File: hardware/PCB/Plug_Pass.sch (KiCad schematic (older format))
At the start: 14 parts, among them J1 Conn_01x06, J10 TDPT-1017503, J2 Conn_01x08, J3 Conn_01x06, J4 QuickDisconnect, J5 Conn_WallSocket_Earth, J6 QuickDisconnect, J7 Conn_01x06, J8 QuickDisconnect, J9 QuickDisconnect

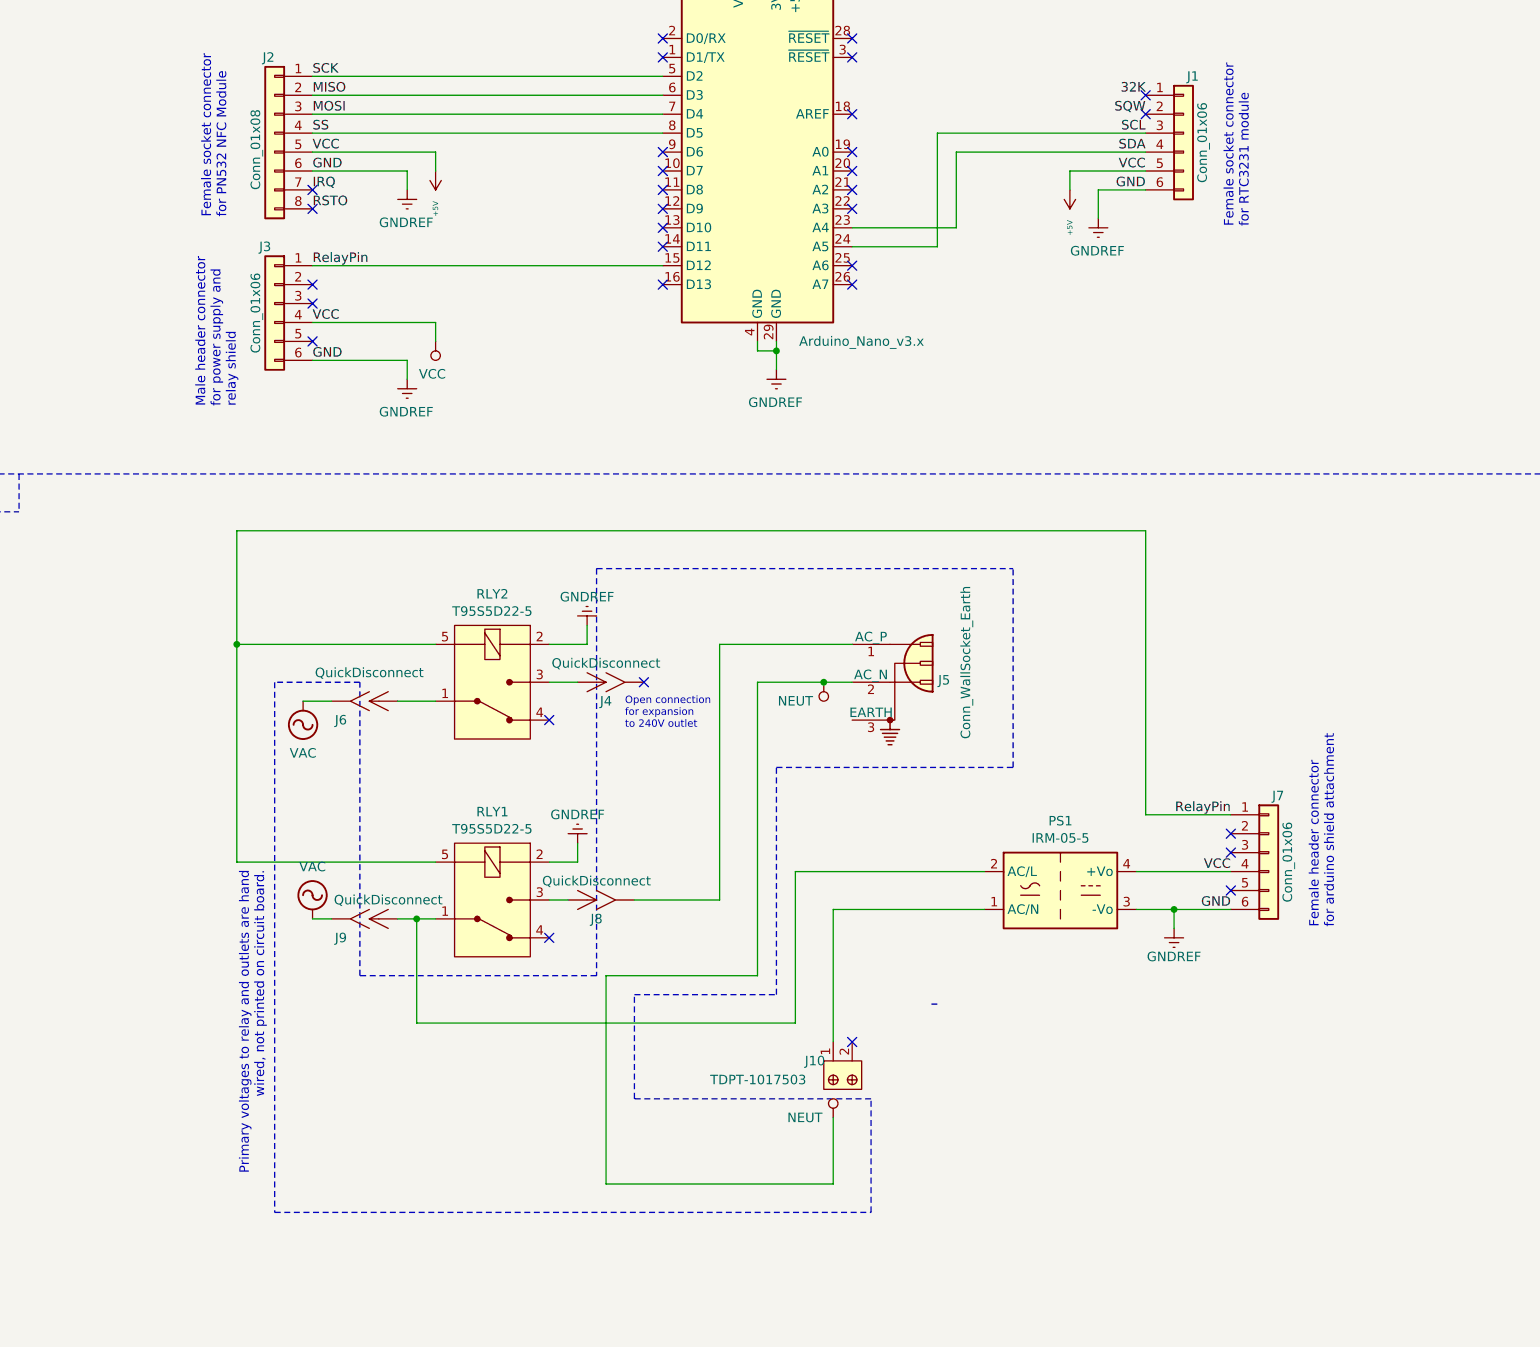
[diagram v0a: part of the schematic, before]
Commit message: Add files via upload
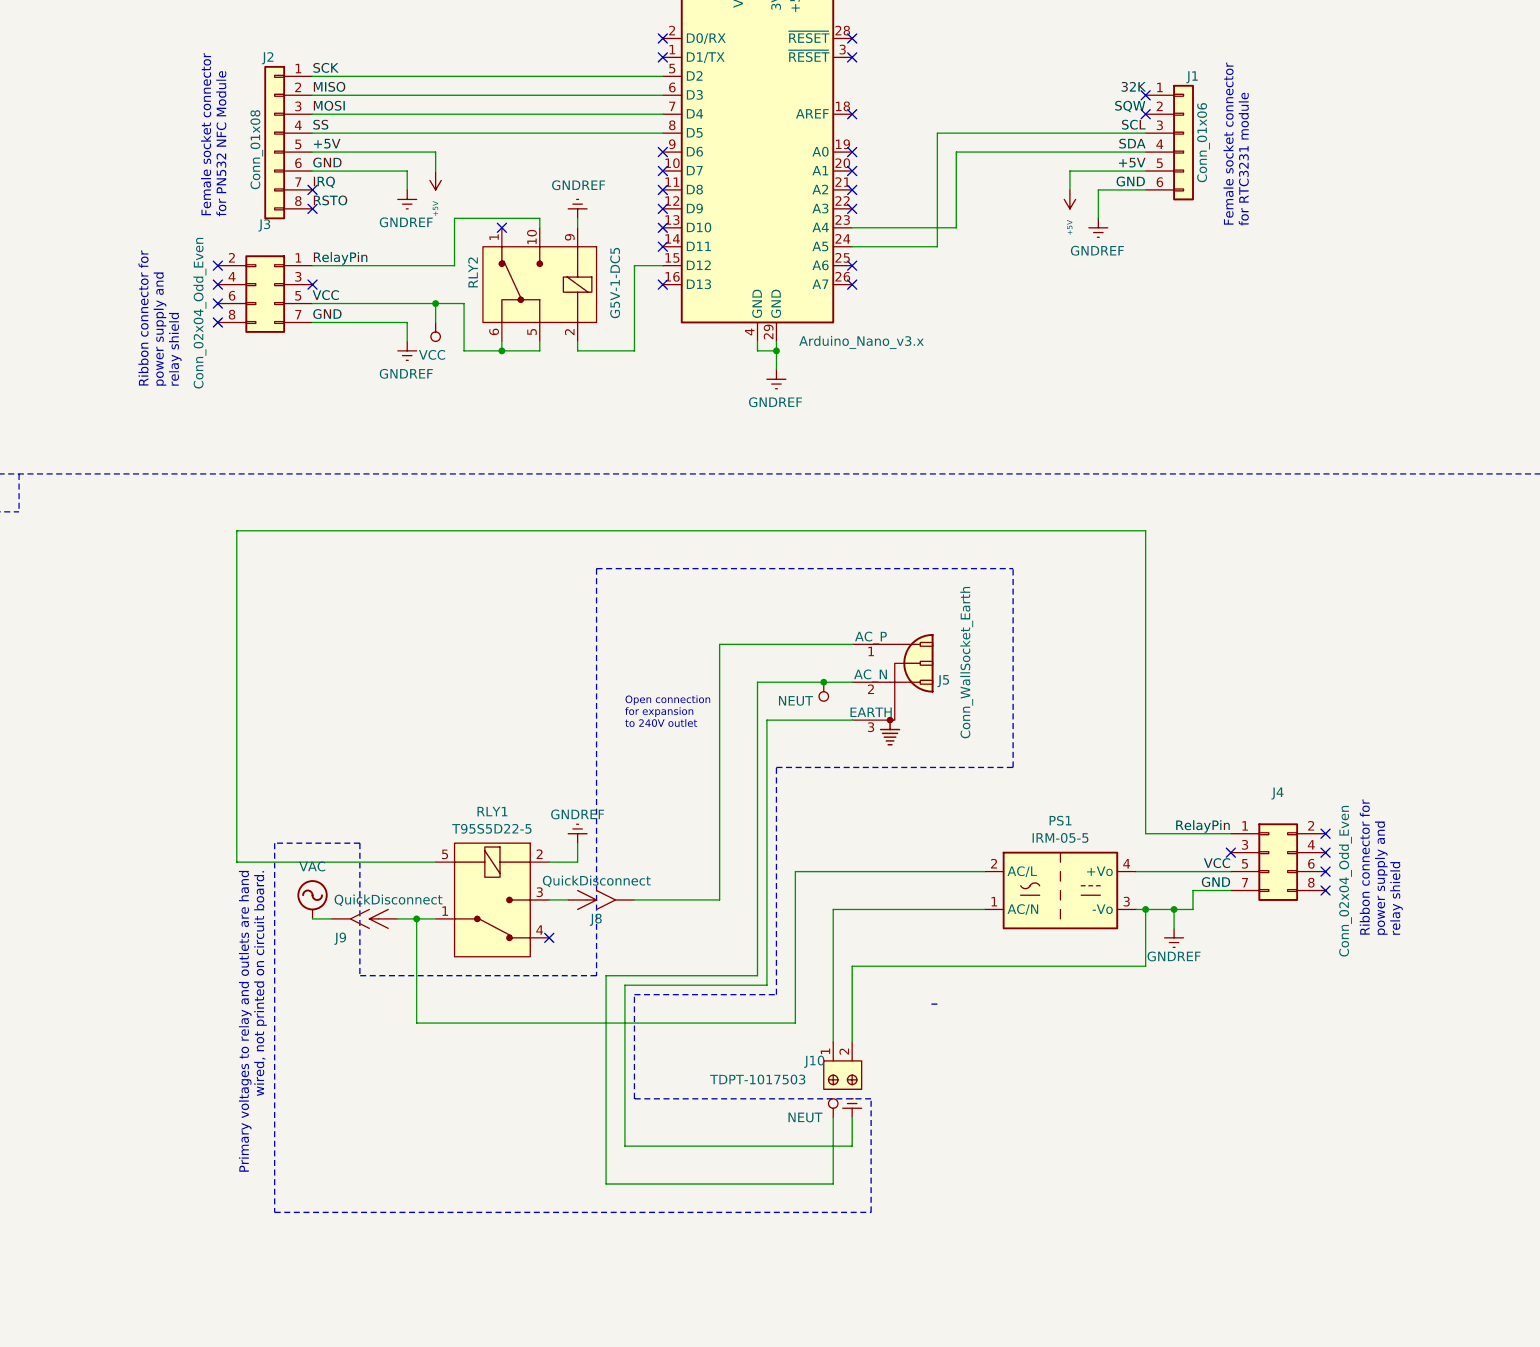
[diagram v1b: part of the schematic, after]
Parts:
- removed J3: Conn_01x06, Plug_Pass:PinHeader_1x06_P2.54mm_Vertical, symbol Plug_Pass:Conn_01x06
- removed J4, J6: QuickDisconnect, symbol Plug_Pass:QuickDisconnect
- removed J7: Conn_01x06, Plug_Pass:PinSocket_1x06_P2.54mm_Vertical, symbol Plug_Pass:Conn_01x06
- removed RLY2: T95S5D22-5, Plug_Pass:RLY-T9AS5D22-5, symbol Plug_Pass:G5LE-14_DC5
- added J3, J4: Conn_02x04_Odd_Even, Plug_Pass:IDC-Header_2x04_P2.54mm_Vertical, symbol Plug_Pass:Conn_02x04_Odd_Even
- added RLY2: G5V-1-DC5, Plug_Pass:Relay_THT_G5V-1, symbol Plug_Pass:G5V-1-DC5
- J10: footprint Plug_Pass:TDPT_2P_5.08MM -> Plug_Pass:TDPT_2P_6.35MM
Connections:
- net +5V: no longer A1.30 (VIN), PS1.4 (+Vo)
- net GNDREF: now also J10.2, J3.7 (Pin_7), J4.7 (Pin_7), RLY2.9 (COIL)
- net RelayPin: now also J3.1 (Pin_1), J4.1 (Pin_1), RLY2.10 (NO); no longer A1.15 (D12)
- net Earth: now reaches J5.3 (EARTH)
- new net: A1.15 (D12), RLY2.2 (COIL)
- new net VCC: A1.30 (VIN), J3.5 (Pin_5), J4.5 (Pin_5), PS1.4 (+Vo), RLY2.5 (COM), RLY2.6 (COM)
- no-connect marks 34 -> 36
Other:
- note added: "Ribbon connector for\npower supply and\nrelay shield"
- note removed: "Female header connector \nfor arduino shield attachment"
- note removed: "Male header connector \nfor power supply and\nrelay shield"
